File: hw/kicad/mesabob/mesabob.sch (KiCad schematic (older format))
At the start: 25 parts, among them J1 RJ45, J2 RJ45, J3 RJ45, J4 RJ45, J5 RJ45, J6 RJ45, J7 RJ45, J8 RJ45, P1 CONN_02X13, U1 rs4854, U2 rs4854, U3 rs4854, U4 rs4854, U5 rs4854, U6 rs4854, U7 rs4854, U8 rs4854

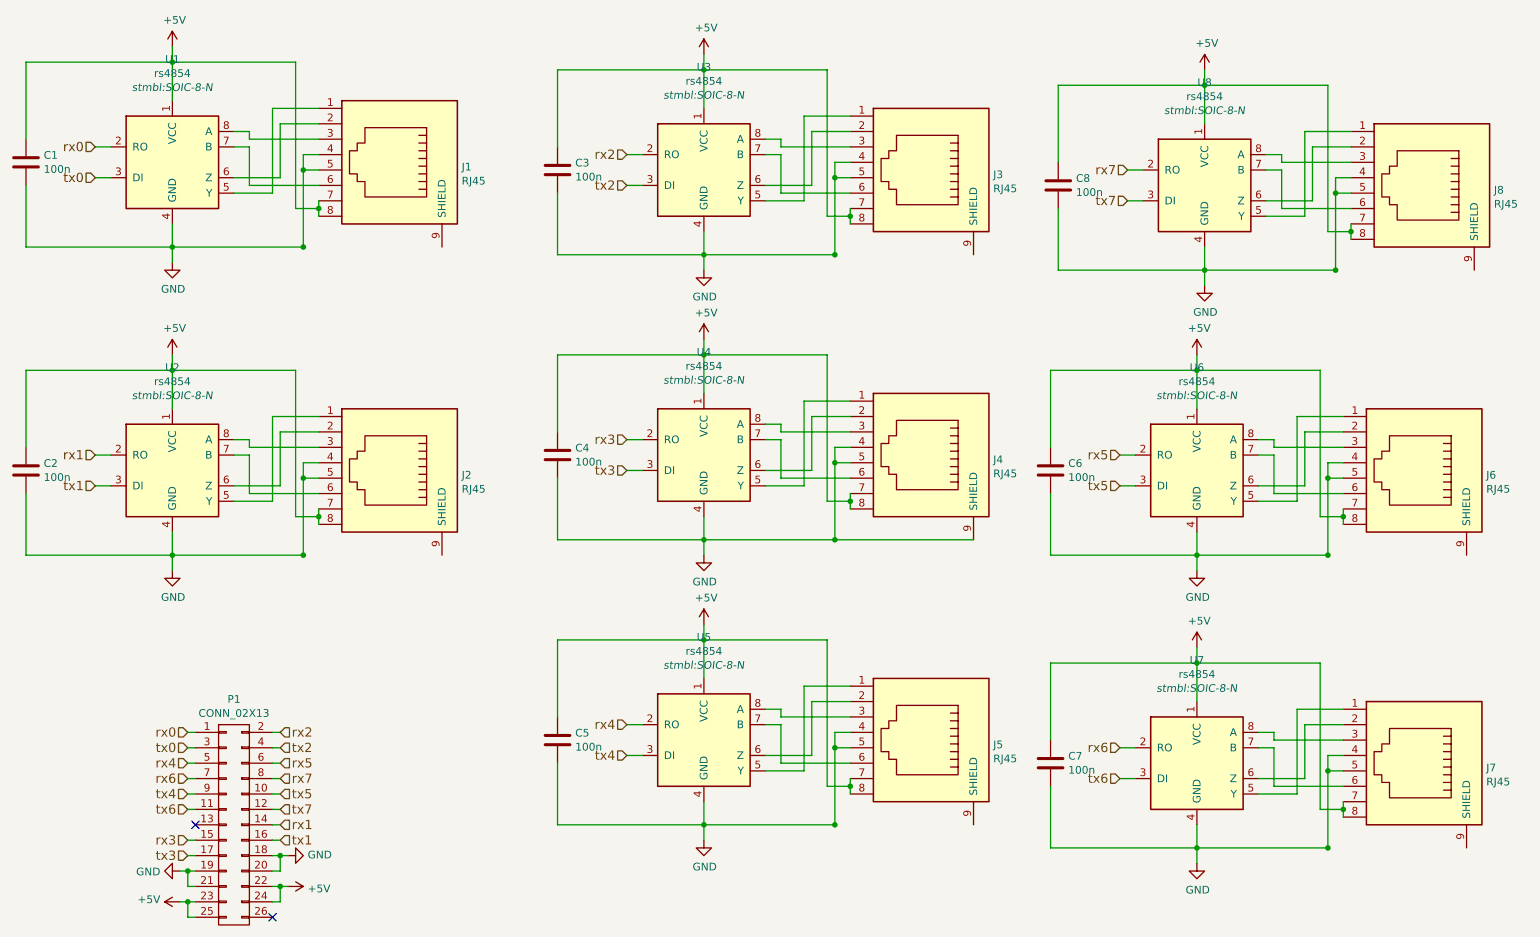
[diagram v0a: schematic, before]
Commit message: mesabob resistors
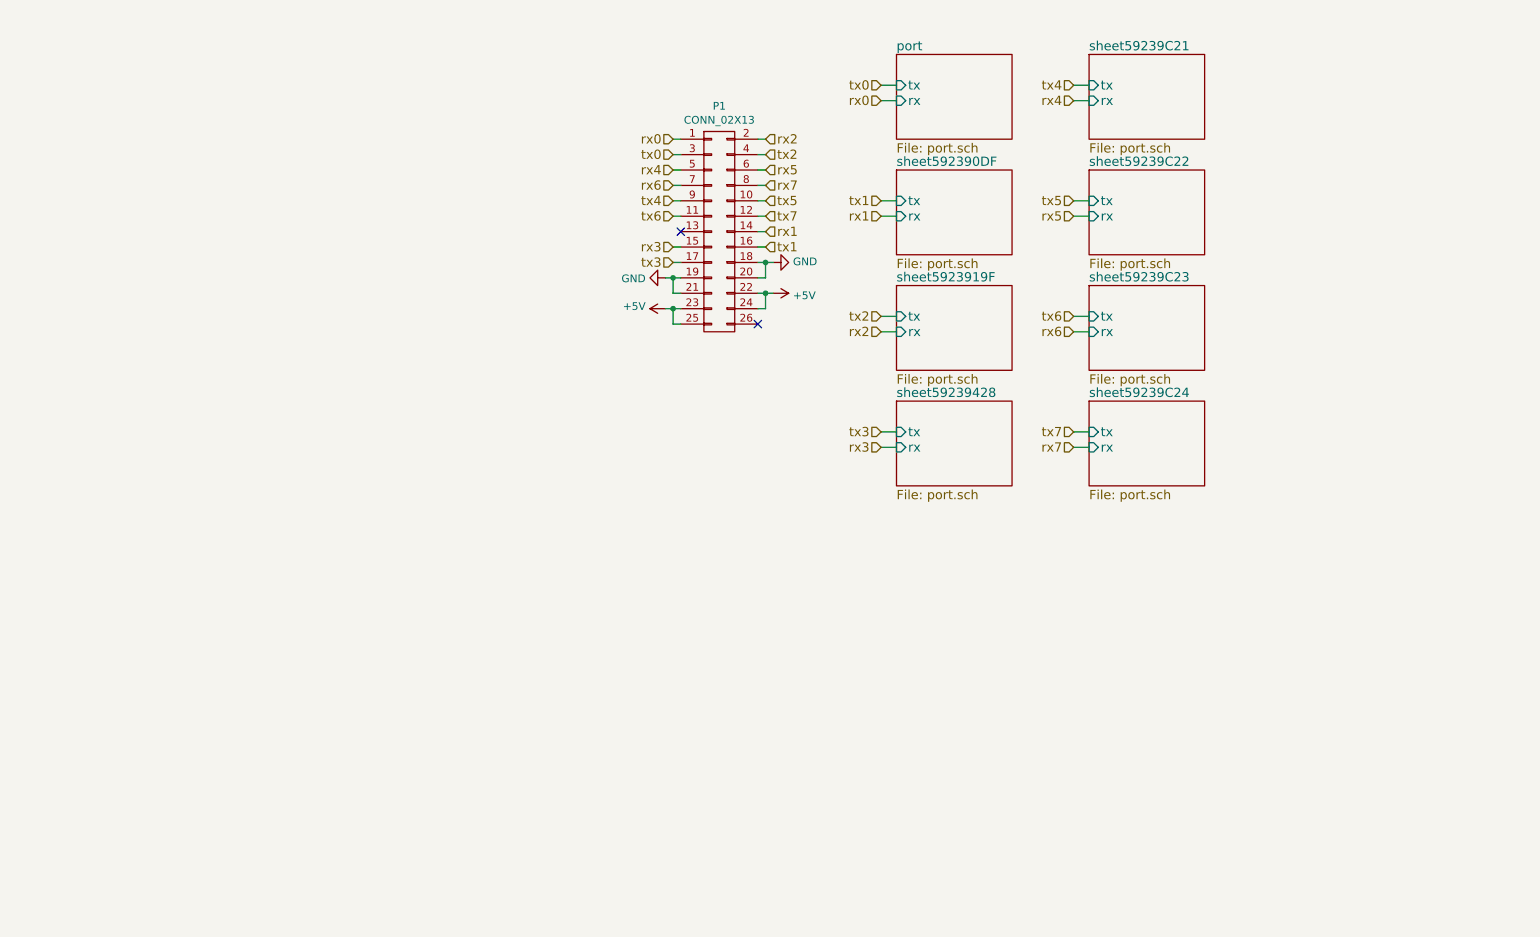
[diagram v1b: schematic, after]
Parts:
- removed C1, C2, C3, C4, C5, C6, C7, C8: 100n, stmbl:C_0603, symbol C
- removed J1, J2, J3, J4, J5, J6, J7, J8: RJ45, Connect:RJ45_8, symbol RJ45
- removed U1, U2, U3, U4, U5, U6, U7, U8: rs4854, stmbl:SOIC-8-N, symbol rs4854
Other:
- moved on the sheet: P1
